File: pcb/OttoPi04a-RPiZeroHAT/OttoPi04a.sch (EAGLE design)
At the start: 26 parts

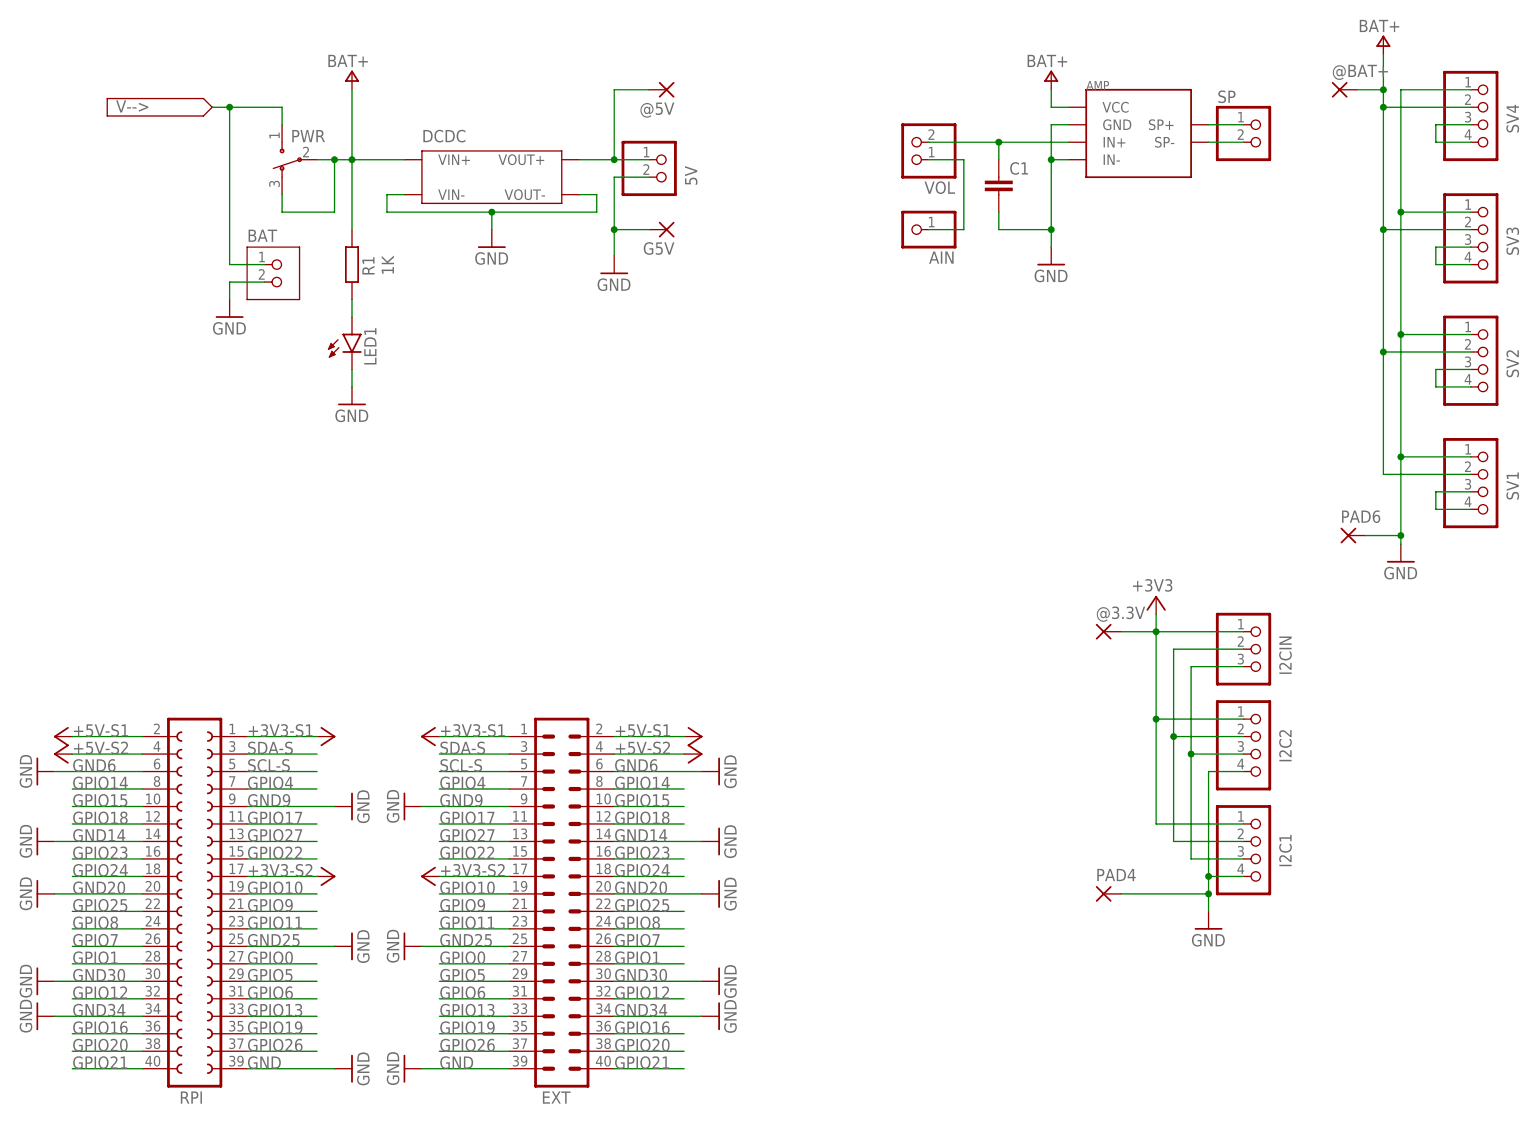
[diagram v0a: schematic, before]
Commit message: update
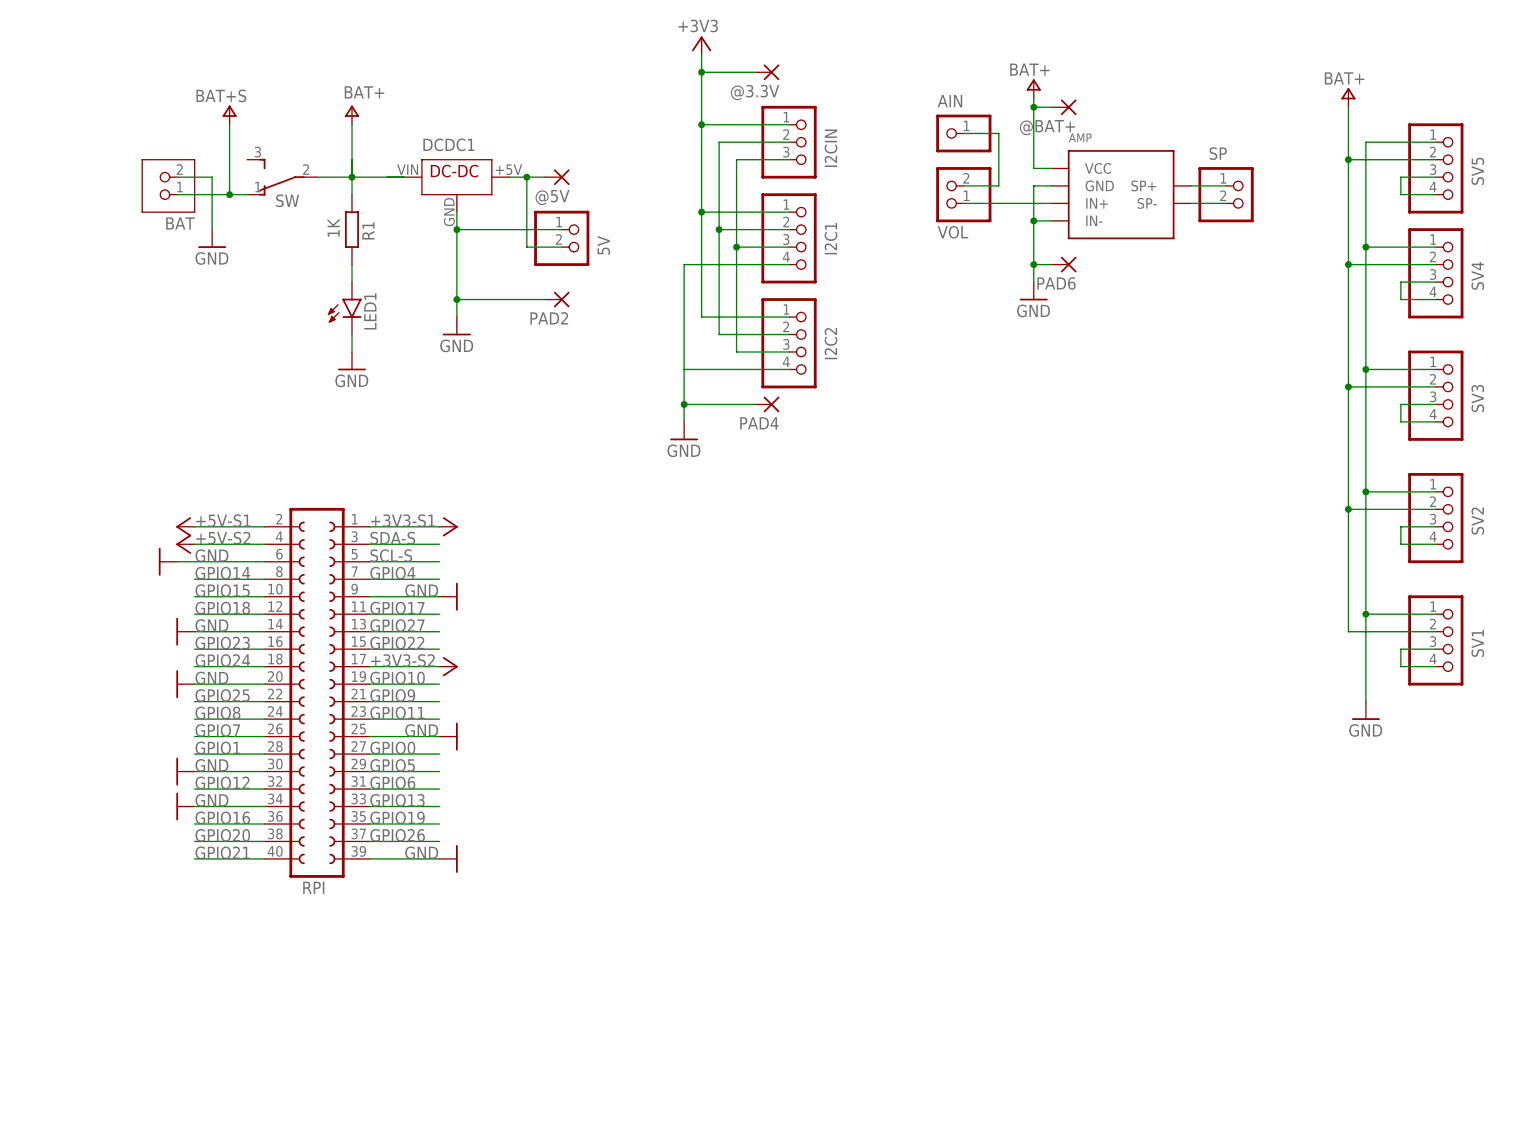
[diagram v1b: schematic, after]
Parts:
- removed C1: (no value), rcl:C-EU025-024X044
- removed DCDC: (no value), ytani1:DCDC-5V_28V-2A
- removed EXT: (no value), con-lstb:MA20-2W
- removed G5V: (no value), wirepad:2,15/1,0
- removed PWR: (no value), ytani1:SW3-1
- added DCDC1: (no value), ytani1:DCDC-5V-0.48A
- added PAD2: (no value), wirepad:1,6/0,9
- added SV5: (no value), pinhead:PINHD-1X4
- added SW: TL36PO, switch:TL36PO
- @3.3V, @5V, @BAT+, PAD4, PAD6: device wirepad:2,15/1,0 -> wirepad:1,6/0,9
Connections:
- removed net AIN1: AIN.1, VOL.1
- removed net BAT+: @BAT+.P, DCDC.VIN+, PWR.2, PWR.3, R1.2, SV1.2, SV2.2, SV3.2, SV4.2
- removed net BAT+S: BAT.1, PWR.1
- removed net GND14: EXT.14, RPI.14
- removed net GND20: EXT.20, RPI.20
- removed net GND25: EXT.25, RPI.25
- removed net GND30: EXT.30, RPI.30
- removed net GND34: EXT.34, RPI.34
- removed net GND6: EXT.6, RPI.6
- removed net GND9: EXT.9, RPI.9
- new net +4V_S: BAT.1, SW.O
- new net N$1: AIN.1, VOL.2
- new net SV5: SV5.3, SV5.4
- net +3V3-S1: no longer EXT.1
- net +3V3-S2: no longer EXT.17
- net +5V: now also 5V.2, DCDC1.VOUT; no longer 5V.1, DCDC.VOUT+
- net +5V-S1: no longer EXT.2
- net +5V-S2: no longer EXT.4
- net AIN: now also VOL.1; no longer C1.1, VOL.2
- net GND: now also 5V.1, DCDC1.GND, PAD2.P, RPI.14, RPI.20, RPI.25, RPI.30, RPI.34, RPI.6, RPI.9, SV5.1; no longer 5V.2, C1.2, DCDC.VIN-, DCDC.VOUT-, EXT.39, G5V.P
- net GPIO0: no longer EXT.27
- net GPIO1: no longer EXT.28
- net GPIO10: no longer EXT.19
- net GPIO11: no longer EXT.23
- net GPIO12: no longer EXT.32
- net GPIO13: no longer EXT.33
- net GPIO14: no longer EXT.8
- net GPIO15: no longer EXT.10
- net GPIO16: no longer EXT.36
- net GPIO17: no longer EXT.11
- net GPIO18: no longer EXT.12
- net GPIO19: no longer EXT.35
- net GPIO20: no longer EXT.38
- net GPIO21: no longer EXT.40
- net GPIO22: no longer EXT.15
- net GPIO23: no longer EXT.16
- net GPIO24: no longer EXT.18
- net GPIO25: no longer EXT.22
- net GPIO26: no longer EXT.37
- net GPIO27: no longer EXT.13
- net GPIO4: no longer EXT.7
- net GPIO5: no longer EXT.29
- net GPIO6: no longer EXT.31
- net GPIO7: no longer EXT.26
- net GPIO8: no longer EXT.24
- net GPIO9: no longer EXT.21
- net SCL-S: no longer EXT.5
- net SDA-S: no longer EXT.3
- net V+: now also @BAT+.P, DCDC1.VIN, R1.2, SV1.2, SV2.2, SV3.2, SV4.2, SV5.2, SW.P
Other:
- moved on the sheet: 5V, @3.3V, @5V, @BAT+, AIN, AMP, BAT, I2C1, I2C2, I2CIN, LED1, PAD4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
